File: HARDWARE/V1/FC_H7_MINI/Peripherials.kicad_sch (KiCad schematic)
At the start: 8 parts, among them IC1 ICM-42688-P, IC3 MX25R1635FZUIH0

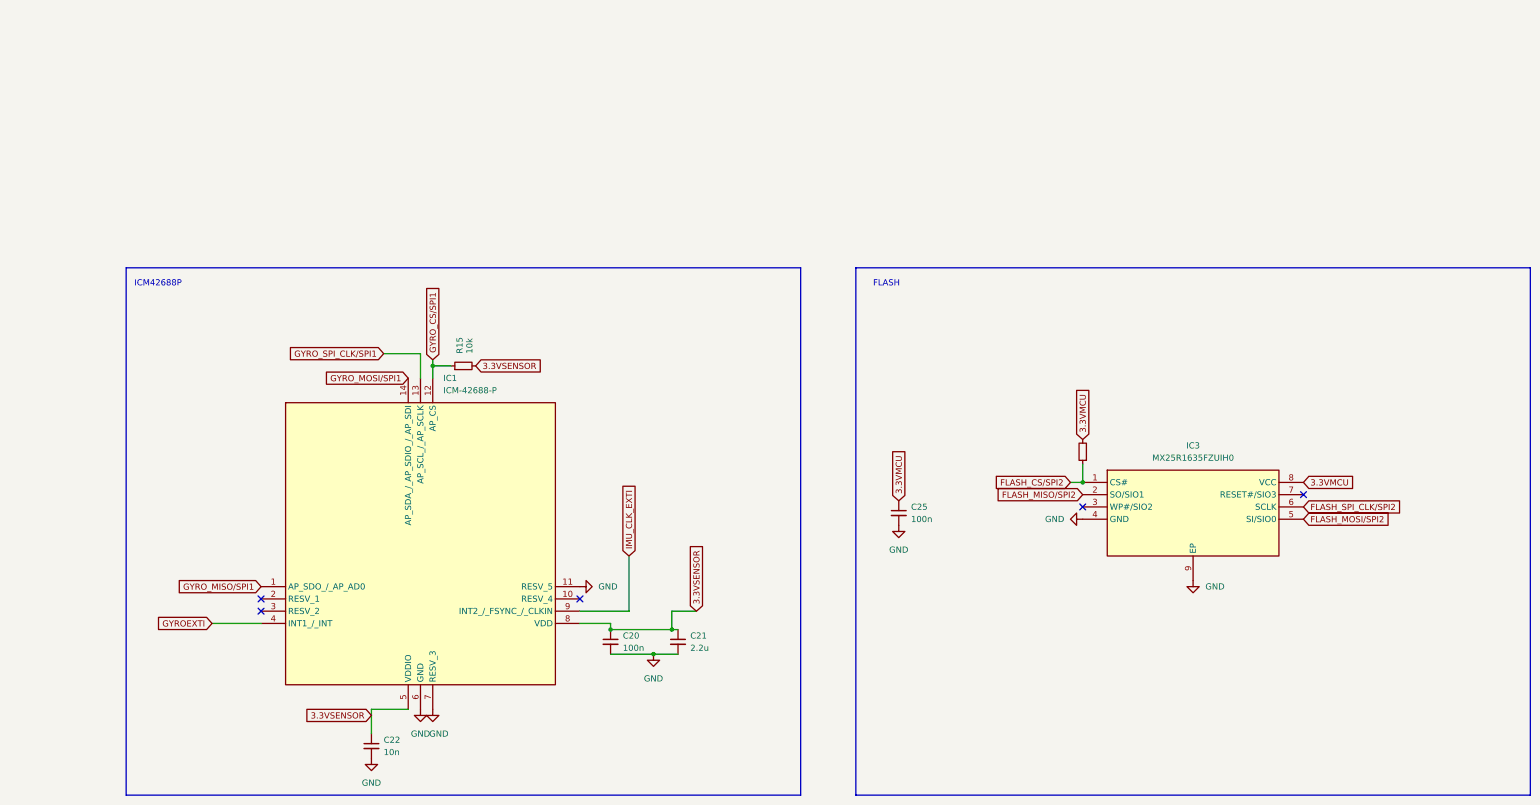
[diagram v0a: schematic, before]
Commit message: up
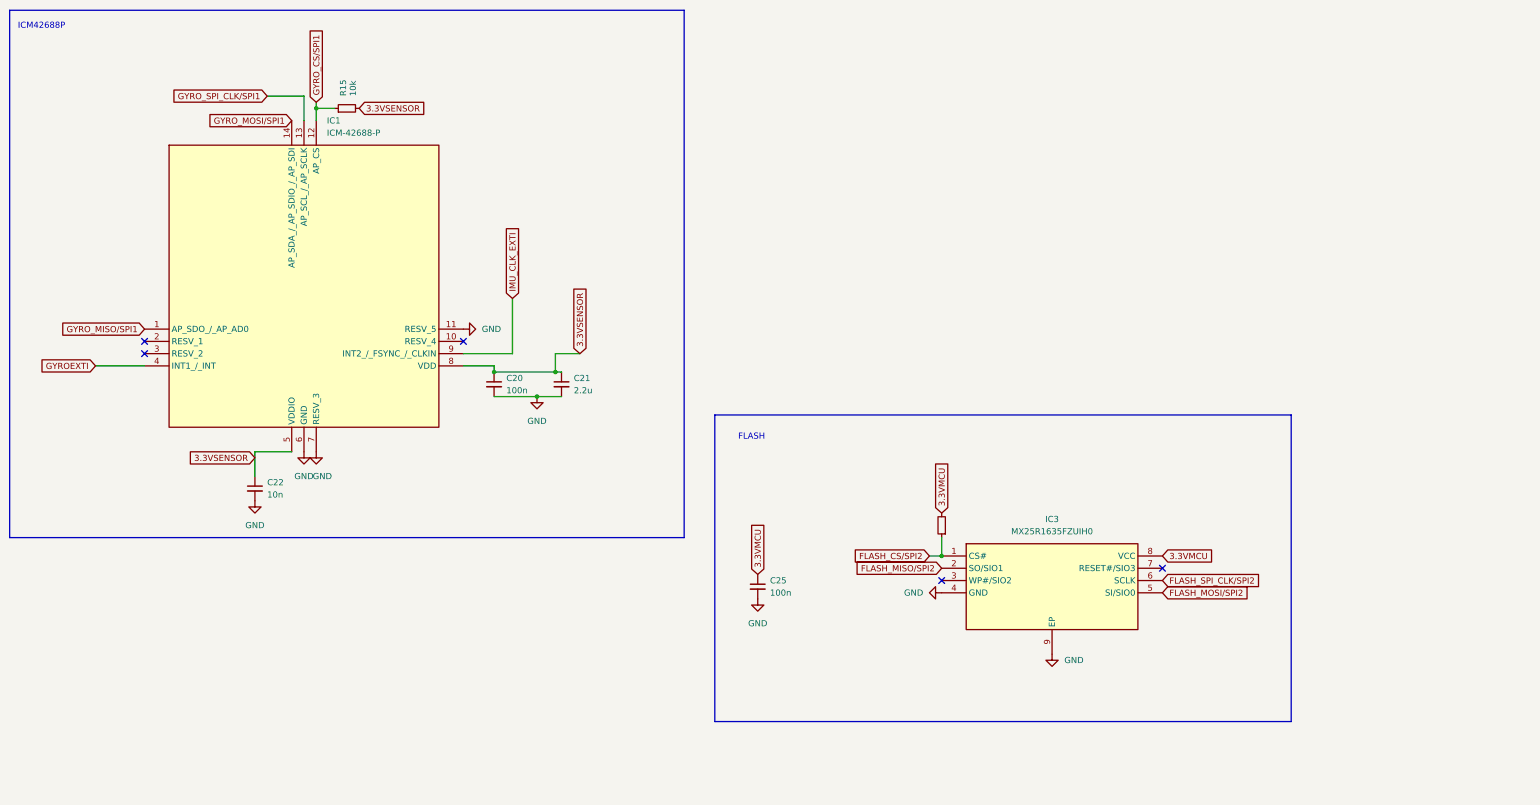
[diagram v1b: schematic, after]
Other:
- moved on the sheet: C20, C21, C22, C25, IC1, IC3, R15
